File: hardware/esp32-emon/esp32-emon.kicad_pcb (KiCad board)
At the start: 2 copper layers, 49.8 x 55.8 mm, 13 parts, among them J1 SJ-3523-SMT-TR, J2 Barrel_Jack, U1 ESP32-DEVKIT-V1

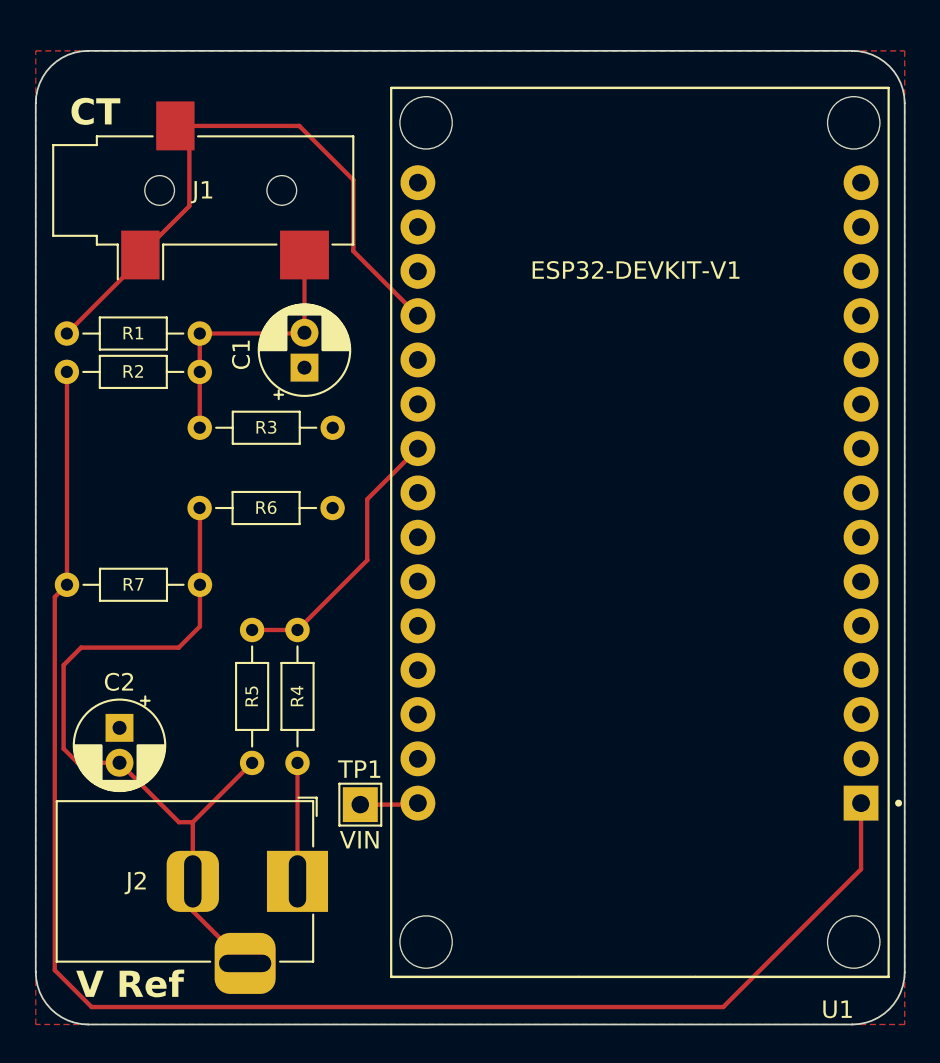
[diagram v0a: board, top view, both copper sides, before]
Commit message: Test TurboCase
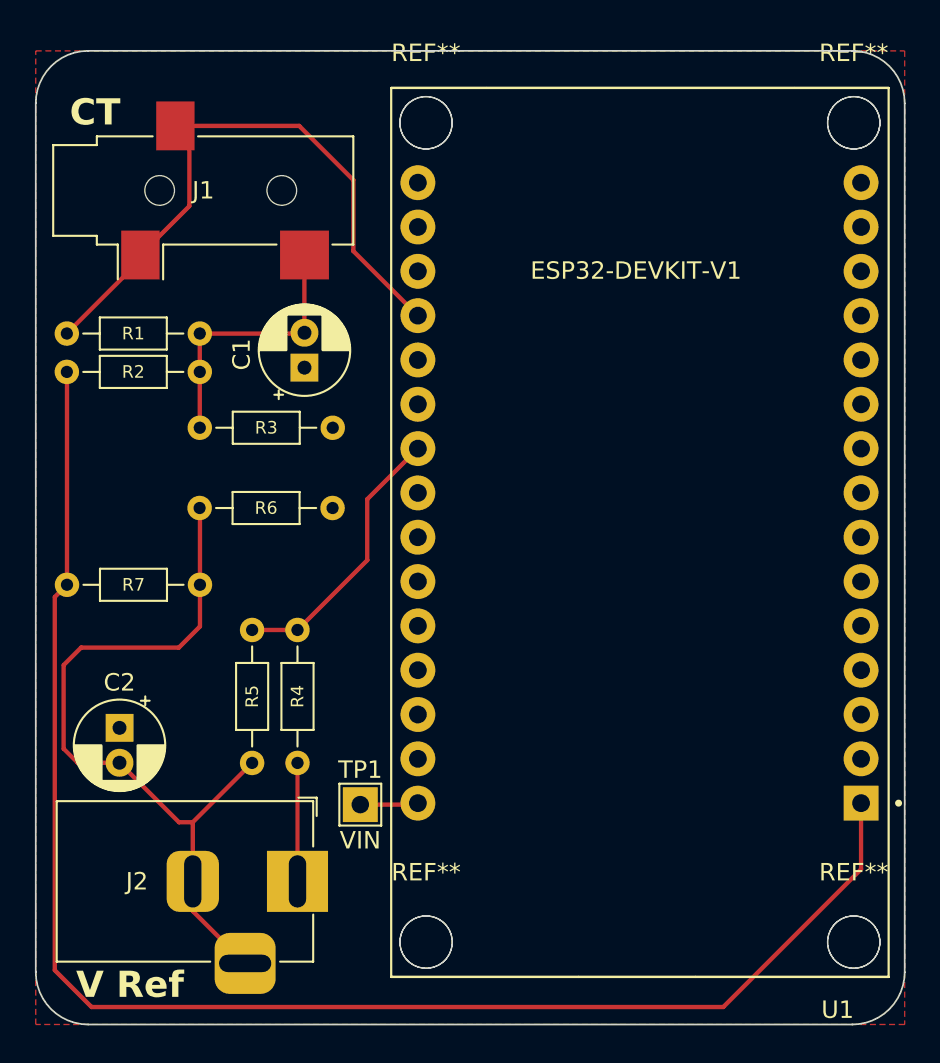
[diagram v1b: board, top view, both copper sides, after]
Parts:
- added ?: , TurboCase:Cutout_Pinheader_01x04_254, F.Cu at (140.8, 34.0)
- added REF**: MountingHole_3mm, MountingHole:MountingHole_3mm, F.Cu at (162.2, 30.1)
- added REF**: MountingHole_3mm, MountingHole:MountingHole_3mm, F.Cu at (186.7, 30.1)
- added REF**: MountingHole_3mm, MountingHole:MountingHole_3mm, F.Cu at (162.2, 77.1)
- added REF**: MountingHole_3mm, MountingHole:MountingHole_3mm, F.Cu at (186.7, 77.1)
